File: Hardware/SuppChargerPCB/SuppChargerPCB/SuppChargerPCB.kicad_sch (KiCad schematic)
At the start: 35 parts, among them J1 SLIMSTACK, J2 SLIMSTACK, Q1 NMOS, Q2 NMOS, Q3 NMOS, Q4 NMOS, U1 BQ25756ERRVR

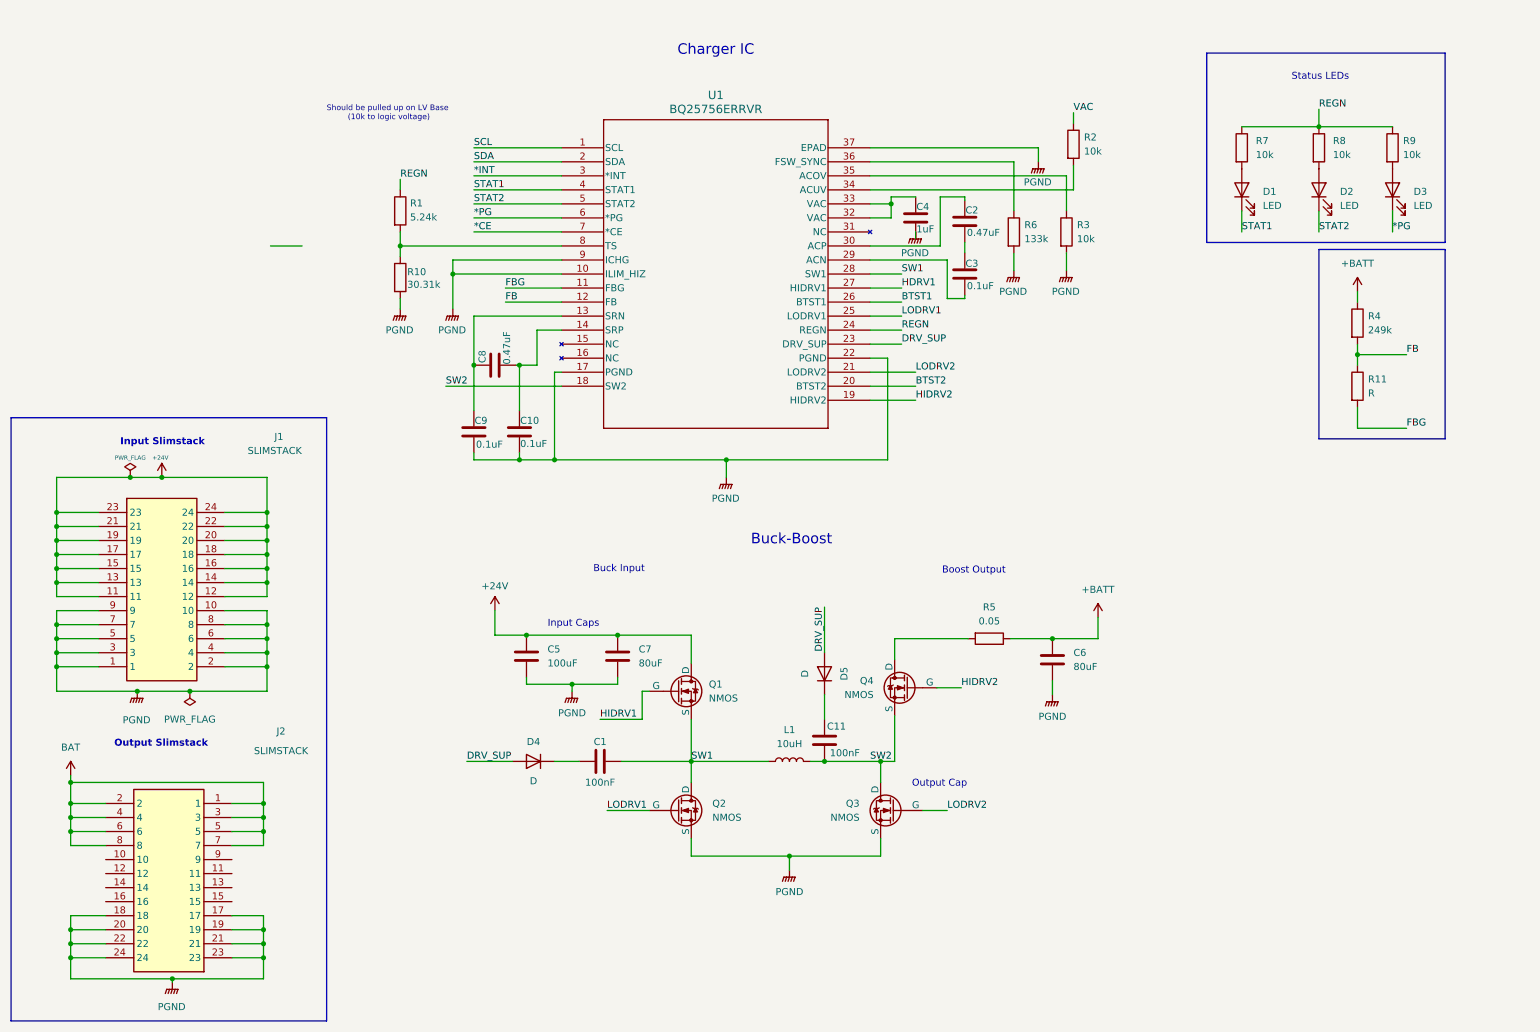
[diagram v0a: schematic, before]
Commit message: need to add connector symbols, desmos
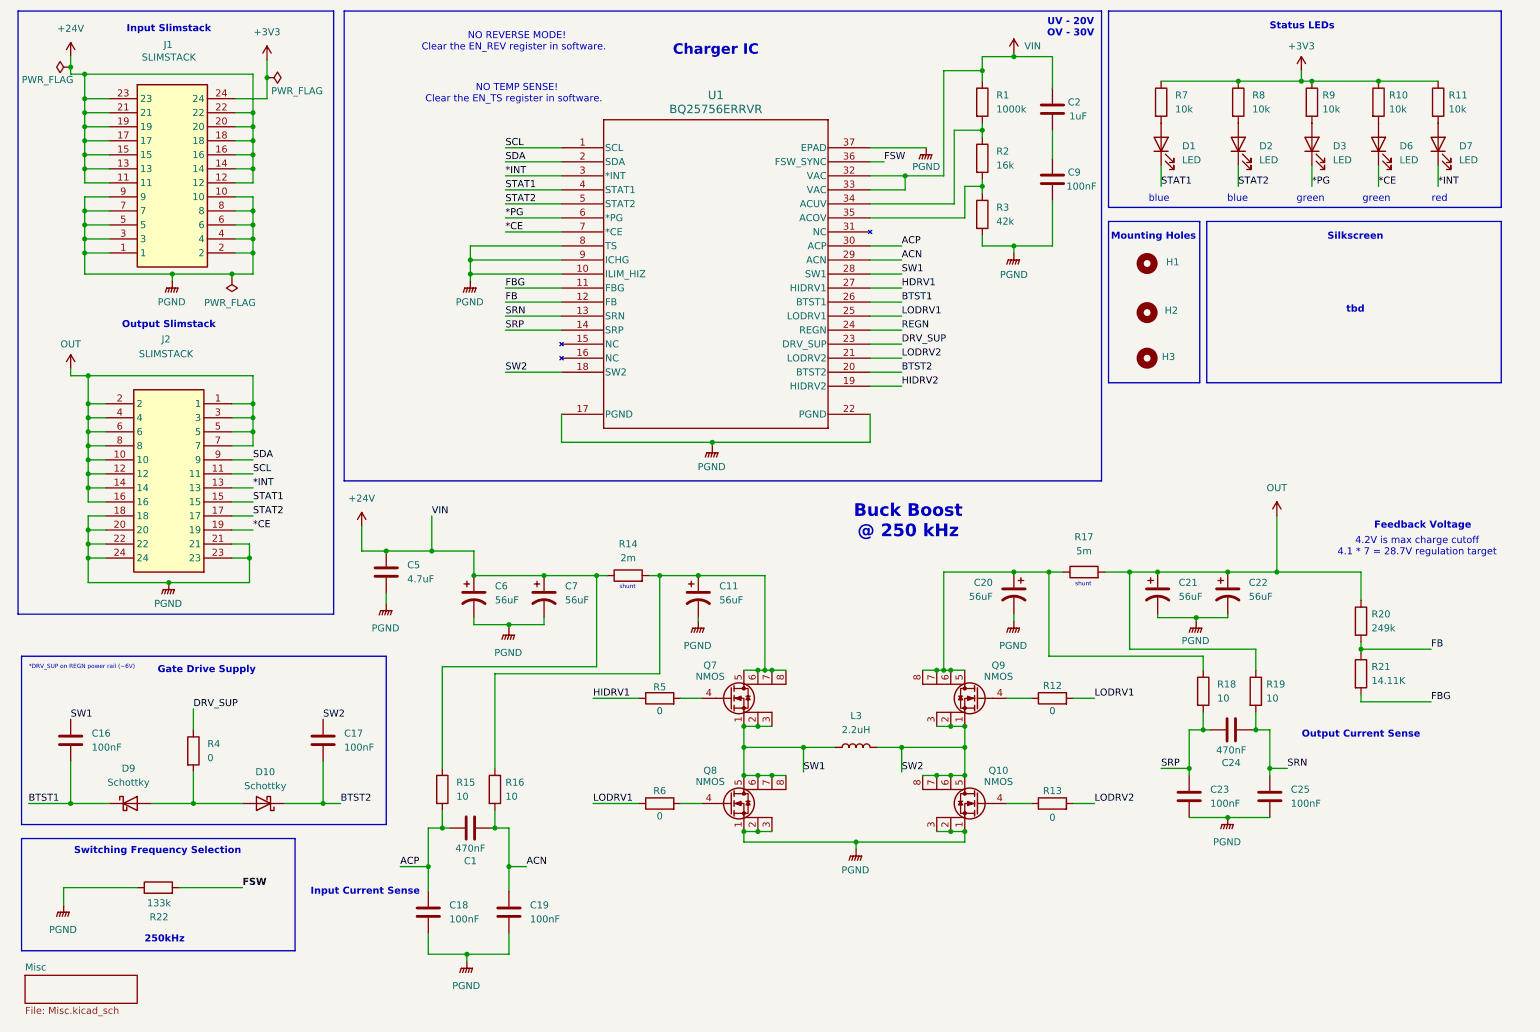
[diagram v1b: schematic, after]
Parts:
- removed C10, C3: 0.1uF, symbol Device:C
- removed C11: 100nF, symbol Device:C
- removed C4: 1uF, symbol Device:C
- removed C6, C7: 80uF, symbol Device:C
- removed C8: 0.47uF, symbol Device:C
- removed D4, D5: D, symbol Device:D
- removed L1: 10uH, symbol Device:L
- removed Q1, Q2, Q3, Q4: NMOS, symbol Simulation_SPICE:NMOS
- added C11, C20, C21, C22, C6, C7: 56uF, symbol Device:C_Polarized_US
- added C16, C17, C18, C19, C23, C25: 100nF, symbol Device:C
- added C24: 470nF, symbol Device:C
- added D10, D9: Schottky, symbol Device:D_Schottky
- added D6, D7: LED, symbol Device:LED
- added H1, H2, H3: MountingHole, symbol Mechanical:MountingHole
- added L3: 2.2uH, symbol Device:L
- added Q10, Q7, Q8, Q9: NMOS, symbol NMOS_Buck:SI3456DDV-T1-GE3
- added R12, R13: 0, symbol Device:R
- added R14: 2m, symbol Device:R
- added R15, R16, R18, R19: 10, symbol Device:R
- added R17: 5m, symbol Device:R
- added R20: 249k, symbol Device:R
- added R21: 14.11K, symbol Device:R
- added R22: 133k, symbol Device:R
- C1: value 100nF -> 470nF
- C2: value 0.47uF -> 1uF
- C5: value 100uF -> 4.7uF
- C9: value 0.1uF -> 100nF
- R1: value 5.24k -> 1000k
- R10: value 30.31k -> 10k
- R11: value R -> 10k
- R2: value 10k -> 16k
- R3: value 10k -> 42k
- R4: value 249k -> 0
- R5: value 0.05 -> 0
- R6: value 133k -> 0
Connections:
- net BAT is gone; now on net OUT: J2.1, J2.2, J2.3, J2.4, J2.5, J2.6, J2.7, J2.8
- net VAC is gone; now on an unnamed net: R2.1
- net *CE: now also J2.19, D6.1 (K)
- net *INT: now also J2.13, D7.1 (K)
- net +24V: now also C2.1, R1.1, U1.32 (VAC), U1.33 (VAC), C6.1, C7.1, R14.1, R15.1; no longer J1.24
- net BTST1: now also C16.2, D9.1 (K)
- net BTST2: now also C17.2, D10.1 (K)
- net DRV_SUP: now also R4.1
- net FB: now also R20.2, R21.1; no longer R11.1, R4.2
- net FBG: now also R21.2; no longer R11.2
- net HIDRV1: now also R5.1
- net LODRV1: now also R6.1, R12.2
- net LODRV2: now also R13.2
- net PGND: now also U1.8 (TS), C11.2, C18.2, C19.2, C20.2, C21.2, C22.2, C23.2, C25.2, C6.2, C7.2, Q10.1 (S), Q10.2 (S), Q10.3 (S), Q8.1 (S), Q8.2 (S), Q8.3 (S), R22.1; no longer J2.17, J2.19, R10.2, R6.2
- net REGN: no longer R1.1, R7.1, R8.1, R9.1
- net SCL: now also J2.11
- net SDA: now also J2.9
- net STAT1: now also J2.15
- net STAT2: now also J2.17
- net SW1: now also C16.1, L3.1, Q7.1 (S), Q7.2 (S), Q7.3 (S), Q8.5 (D), Q8.6 (S), Q8.7 (S), Q8.8 (S); no longer C1.1
- net SW2: now also C17.1, L3.2, Q10.5 (D), Q10.6 (S), Q10.7 (S), Q10.8 (S), Q9.1 (S), Q9.2 (S), Q9.3 (S)
- net at C9.1: now also C2.2; no longer U1.13 (SRN)
- net at R5.2: now also Q7.4 (G)
- net ACP: now reaches C1.2
- net ACP: now also U1.30 (ACP), C18.1, R15.2
- net FSW: now reaches U1.36 (FSW_SYNC)
- net FSW: now also R22.2; no longer R6.1
- net ACN: now reaches U1.29 (ACN)
- net ACN: now also C1.1, C19.1, R16.2
- net SRP: now reaches U1.14 (SRP)
- net SRP: now also C23.1, C24.2, R18.2
- net OUT: now reaches J2.10
- net OUT: now also J2.12, J2.14, J2.16, C21.1, C22.1, R17.2, R19.1, R20.1
- net at U1.34 (ACUV): now also R1.2; no longer R2.2
- net at R3.1, U1.35 (ACOV): now also R2.2
- removed net +BATT: R4.1, R5.1
- new net: C11.1, Q7.5 (D), Q7.6 (S), Q7.7 (S), Q7.8 (S), R14.2, R16.1
- new net: C20.1, Q9.5 (D), Q9.6 (S), Q9.7 (S), Q9.8 (S), R17.1, R18.1
- new net: Q10.4 (G), R13.1
- new net: D6.2 (A), R10.2
- new net: D10.2 (A), D9.2 (A), R4.2
- new net: Q9.4 (G), R12.1
- new net: Q8.4 (G), R6.2
- new net: D7.2 (A), R11.2
- new net +3V3: J1.24, R10.1, R11.1, R7.1, R8.1, R9.1
- new net SRN: C24.1, C25.1, R19.2, U1.13 (SRN)
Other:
- added sheet Misc (Misc.kicad_sch)
- note added: "*DRV_SUP on REGN power rail (~6V)"
- note added: "250kHz"
- note added: "4.2V is max charge cutoff 4.1 * 7 = 28.7V regulation target"
- note added: "Buck Boost @ 250 kHz"
- note added: "Feedback Voltage"
- note added: "Gate Drive Supply"
- note added: "Input Current Sense"
- note added: "Mounting Holes"
- note added: "NO REVERSE MODE! Clear the EN_REV register in software."
- note added: "NO TEMP SENSE! Clear the EN_TS register in software."
- note added: "Output Current Sense"
- note added: "Silkscreen"
- note added: "Switching Frequency Selection"
- note added: "UV - 20V OV - 30V"
- note added: "blue"
- note added: "green"
- note added: "red"
- note added: "shunt"
- note added: "tbd"
- note removed: "Boost Output"
- note removed: "Buck Input"
- note removed: "Buck-Boost"
- note removed: "Input Caps"
- note removed: "Output Cap"
- note removed: "Should be pulled up on LV Base (10k to logic voltage)"
- title: (none) -> Supp Charger
- moved on the sheet: D1, D2, D3, J1, J2, R7, R8, R9
